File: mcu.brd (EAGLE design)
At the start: 35.5 x 57 mm, 63 parts, among them IC1 MCP73831/OT, T1 SI7051-A20, U4 NRF52832, U7 CP2102N-A01-GQFN24, X1 LFXTAL069526, X6 32.768kHz

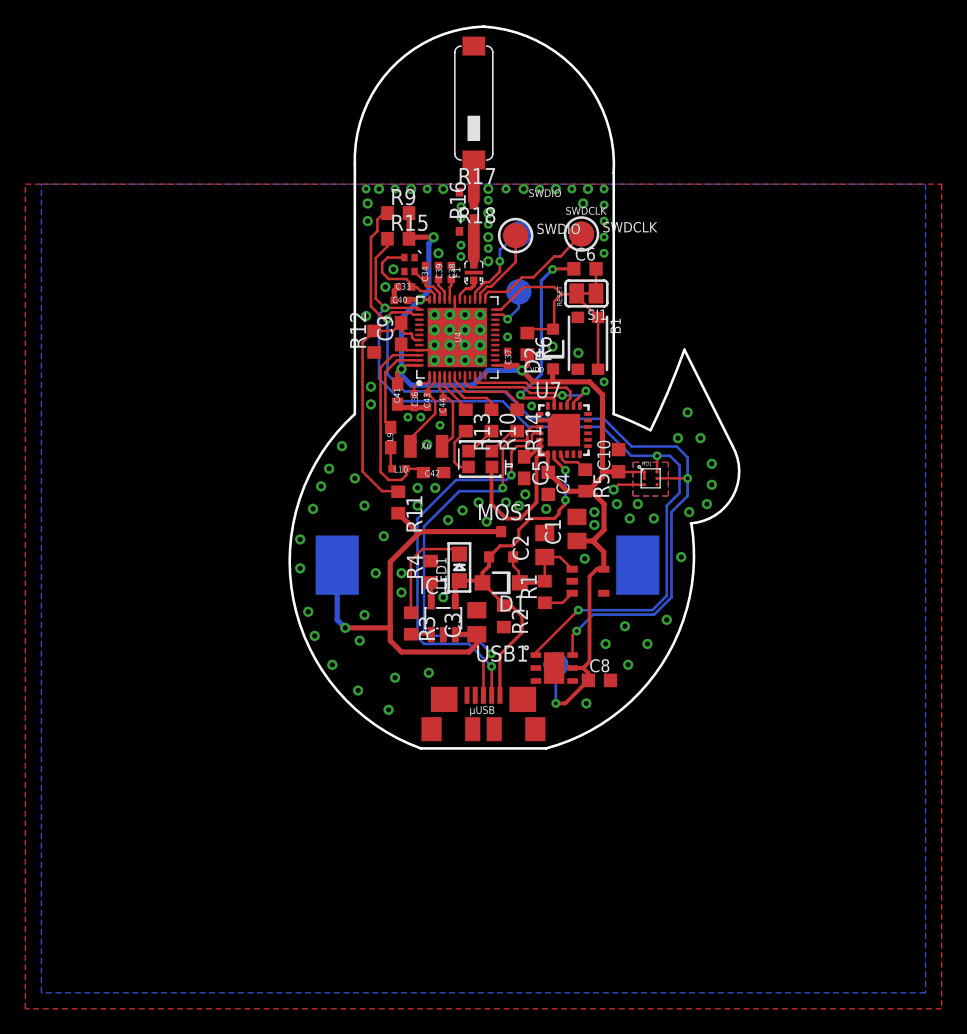
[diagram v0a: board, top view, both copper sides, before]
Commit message: UPD: v2 wiring complete
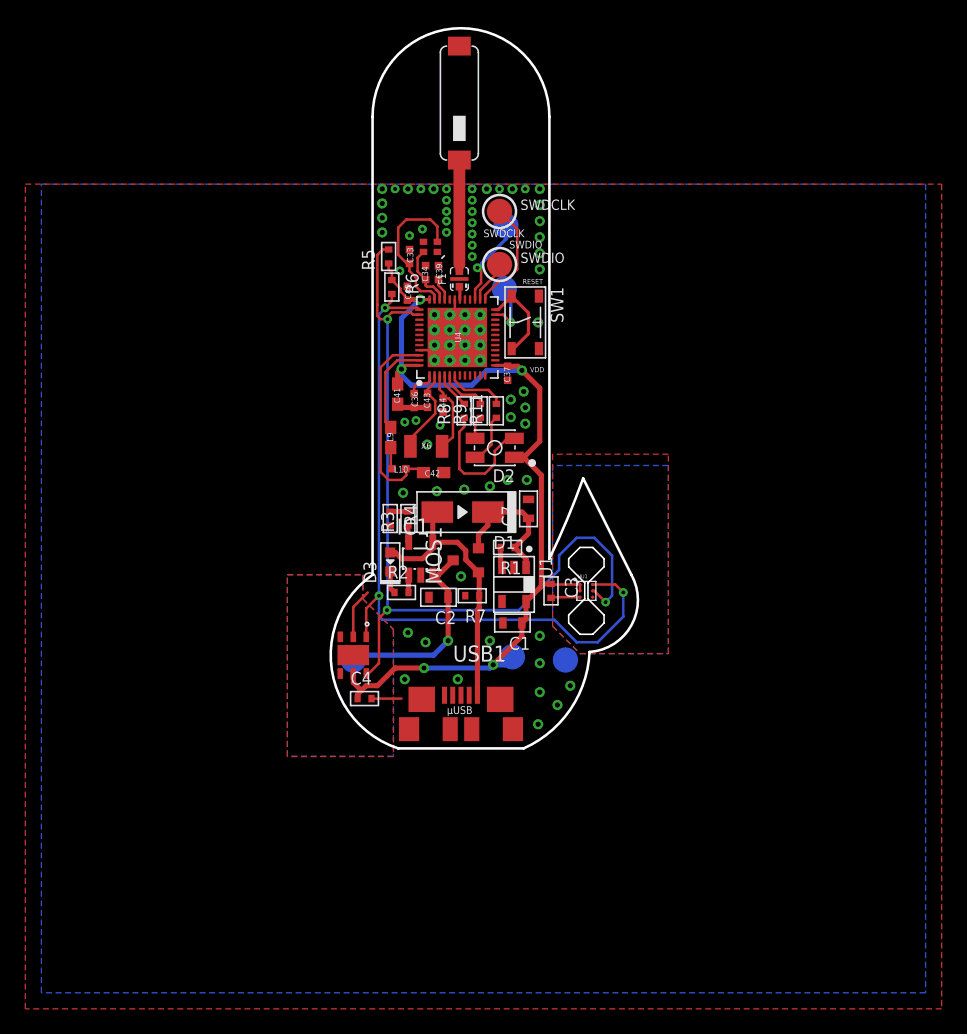
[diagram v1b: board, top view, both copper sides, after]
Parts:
- removed B1: (no value), microbuilder:BTN_KMR2_4.6X2.8
- removed C10, C6, C8: 0.1µF, rcl:C0603K
- removed C38: DNP, Nordic_nRF:RESC0402_N
- removed C5: 4.7µF, rcl:C0603
- removed C9: 1nF, rcl:C0603
- removed LDO1: AP2112-3.3K, tilesPartComp:SOT25
- removed LED1: Orange, microbuilder:CHIPLED_0805
- removed R10, R14: 22, rcl:R0603
- removed R12: 2M, rcl:R0603
- removed R13: 100, rcl:R0603
- removed R15: 10K, rcl:R0603
- removed R16: 0, rcl:R0402
- removed R17, R18: DNP, rcl:R0402
- removed RGB1: 150080M153000, tilesPartComp:RGBLED_0805
- removed SJ1: (no value), microbuilder:SOLDERJUMPER_CLOSEDWIRE
- removed SWO: (no value), microbuilder:TESTPOINT_ROUND_2MM
- removed TEST1, TEST2: TESTPOINT_SQUARE_SMT, tilesPartComp:TESTPOINT_SMT
- removed U7: CP2102N-A01-GQFN24, tilesPartComp:QFN-24
- added BAT+, BAT-, VDD: (no value), microbuilder:TESTPOINT_ROUND_2MM
- added C7: 10uF, MF_Passives:C0603
- added D3: MF-LED-0603-RED, MF_LEDs:LED0603
- added R7: 100K, MF_Passives:R0402
- added R8: 100, MF_Passives:R0402
- added SW1: MF-SW-TACT-4.2MM, MF_Switches:TACT4.2MM
- added U1: MF-REG-SOT235-3.3V-300mA, MF_IC_Power:SOT-23-5
- C1, C2: value 10µF -> 10uF; device rcl:C0805 -> MF_Passives:C0603
- C3: value 10µF -> 0.1uF; device rcl:C0805 -> MF_Passives:C0402
- C4: value 0.1µF -> 0.1uF; device rcl:C0603K -> MF_Passives:C0402
- D1: value NRVB120VLSF -> MF-DIO-SMA-B140; device tilesPartComp:SOD123FL -> MF_Discrete_Semiconductor:SMA
- D2: value 1N4148 -> MF-LED-3228-RGB; device tilesPartComp:SOD123 -> MF_LEDs:PLCC4
- R1, R6: device rcl:R0603 -> MF_Passives:R0402
- R11: value 806K -> 22; device rcl:R0603 -> MF_Passives:R0402
- R2: value 100K -> 560; device rcl:R0603 -> MF_Passives:R0402
- R3: value 200 -> 18K; device rcl:R0603 -> MF_Passives:R0402
- R4: value 37K -> 18K; device rcl:R0603 -> MF_Passives:R0402
- R5: value 1K -> 10K; device rcl:R0603 -> MF_Passives:R0402
- R9: value 10K -> 22; device rcl:R0603 -> MF_Passives:R0402
- moved R5 23.5 mm to (45.2, 60.7), turned to 90 degrees
- moved C4 22.4 mm to (43.3, 25.8), turned to 0 degrees
- moved R9 16.9 mm to (52.5, 48.5), turned to 90 degrees
- moved T1 15.9 mm to (42.4, 29.2), turned to 270 degrees
- moved R6 11.6 mm to (45.5, 58.3)
- moved R11 10.6 mm to (53.7, 48.5), turned to 90 degrees
- moved HU1 10.2 mm to (60.8, 34.3)
- moved C2 9.36 mm to (49.1, 33.8), turned to 180 degrees
- moved D2 9.06 mm to (53.6, 45.6), turned to 180 degrees
- moved C1 9.01 mm to (55.0, 31.8), turned to 180 degrees
- moved R2 8.31 mm to (46.2, 34.2), turned to 0 degrees
- moved R3 8.30 mm to (46.7, 40.0), turned to 90 degrees
- moved SWDCLK 6.72 mm to (54.0, 64.3)
- moved D1 6.37 mm to (51.1, 40.5)
- moved C3 6.36 mm to (58.0, 34.3), turned to 270 degrees
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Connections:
- removed net DTR: C6.1, U7.23
- removed net N$18: ANT1.1, R16.2, R17.2
- removed net N$19: R13.2, RGB1.1
- removed net N$20: R10.2, RGB1.2
- removed net N$21: R14.2, RGB1.3
- new net N$13: R3.P$2, R4.P$1
- new net N$14: D2.P$4, R11.P$1
- net DEC2: no longer C38.1
- net GND: now also BAT-.P$1, C1.P$2, C2.P$2, C3.P$2, C4.P$2, C7.P$2, R4.P$2, R7.P$2, SW1.P$1, SW1.P$2, U1.P$2; no longer B1.B, B1.B', C1.2, C10.2, C2.2, C3.2, C38.2, C4.2, C5.2, C8.2, C9.1, LDO1.2, R12.1, R17.1, R18.1, R2.2, R4.2, TEST2.T, U7.2, U7.EXP
- net N$1: now also R1.P$2, U1.P$3; no longer LDO1.3, R1.1
- net N$2: now also C7.P$1, D1.CATHODE, R1.P$1, U1.P$1; no longer C2.1, D1.C, LDO1.1, R1.2
- net N$3: now also R2.P$2; no longer R3.2
- net N$4: now also D3.CATHODE, R2.P$1; no longer LED1.C, R3.1
- net N$5: now also D2.P$2, R8.P$1; no longer R5.1, U7.9
- net N$6: now also R3.P$1; no longer R4.1
- net N$7: now also D2.P$3, R9.P$1; no longer C6.2, SJ1.1
- net P0.02: now also R8.P$2; no longer R13.1
- net P0.03: now also R9.P$2; no longer R10.1
- net P0.04: now also R11.P$2; no longer R14.1
- net P0.21/RESET: now also SW1.P$3, SW1.P$4; no longer B1.A, B1.A', D2.A, R6.1, SJ1.2
- net P0.25: now also R6.P$2; no longer R15.1
- net P0.26: now also R5.P$2; no longer R9.1
- net P0.31: no longer C9.2, R11.1, R12.2
- net RF: now also ANT1.1; no longer R16.1, R18.2
- net RXD: no longer U7.21
- net TXD: no longer U7.20
- net USBD+: no longer U7.3
- net USBD-: no longer U7.4
- net V+: now also C1.P$1, C3.P$1, C4.P$1, D2.P$1, R5.P$1, R6.P$1, U1.P$5, VDD.P$1; no longer C1.1, C10.1, C4.1, C5.1, C8.1, D2.C, LDO1.5, R15.2, R5.2, R6.2, R9.2, RGB1.4, SWO.P$1, U7.5, U7.6, U7.7
- net VBAT: now also BAT+.P$1, C2.P$1; no longer C3.1, R11.2, TEST1.T
- net VUSB: now also D1.ANODE, D3.ANODE, R7.P$1; no longer D1.A, LED1.A, R2.1, U7.8
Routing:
- net USBD+: track 32.4 -> 0.00 mm, vias 2 -> 0
- net USBD-: track 32.3 -> 0.00 mm, vias 2 -> 0
- net V+: track 101.1 -> 74.3 mm
- net VBAT: track 37.1 -> 15.9 mm
- net P0.31: track 20.3 -> 0.01 mm
- net DTR: track 16.0 -> 0.00 mm, vias 2 -> 0
- net TXD: track 12.3 -> 0.00 mm, vias 2 -> 0
- net P0.21/RESET: track 19.4 -> 7.07 mm
- net RXD: track 9.51 -> 0.00 mm
- net VUSB: track 30.3 -> 21.7 mm, vias 2 -> 0
- net N$5: track 2.61 -> 10.4 mm
- net P0.25: track 65.7 -> 57.9 mm
- net N$4: track 8.49 -> 1.80 mm
- net RF: track 4.18 -> 8.79 mm
- net N$18: track 4.28 -> 0.00 mm
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- added copper zone on layer 16, net N$11
- added copper zone on layer 1, net N$15
- added copper zone on layer 16, net N$15
- added copper zone on layer 1, net N$16
- removed copper zone on layer 1, net N$11
- removed copper zone on layer 16, net N$12
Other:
- board size 35.5 x 57 mm -> 24.3 x 56.9 mm
- board text added: "TilesTemp v2.0 ISSE-IDI-NTNU Trondheim, NO Francesco Gianni Monica Divitini Welle Design"
- board text removed: "TilesTemp v2.0 ISSE-IDI-NTNU Trondheim Francesco Gianni Monica Divitini Welle Design"
